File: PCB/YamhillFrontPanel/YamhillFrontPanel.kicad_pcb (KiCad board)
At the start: 2 copper layers, 110 x 50 mm, 6 parts

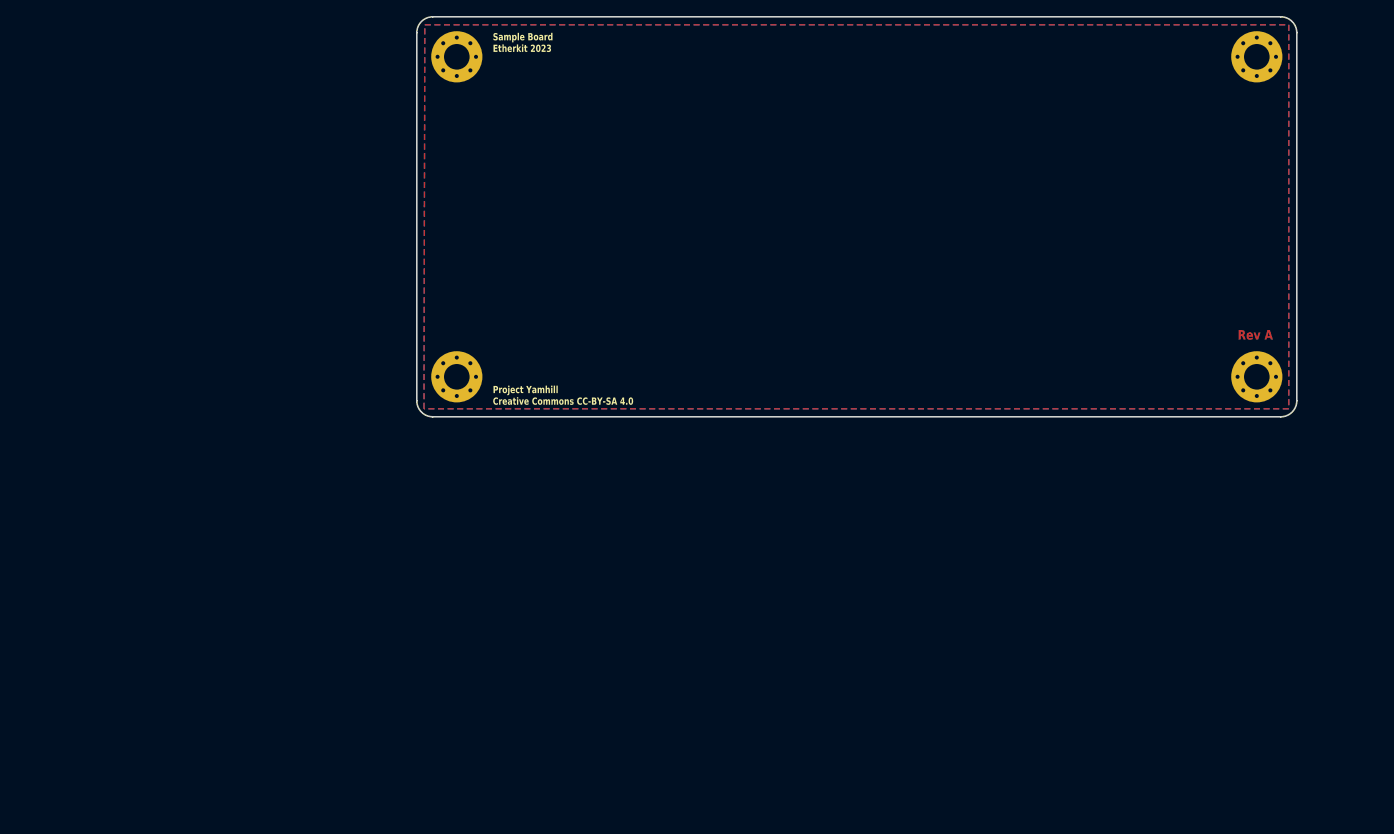
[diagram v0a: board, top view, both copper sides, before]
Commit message: Rev A Front Panel
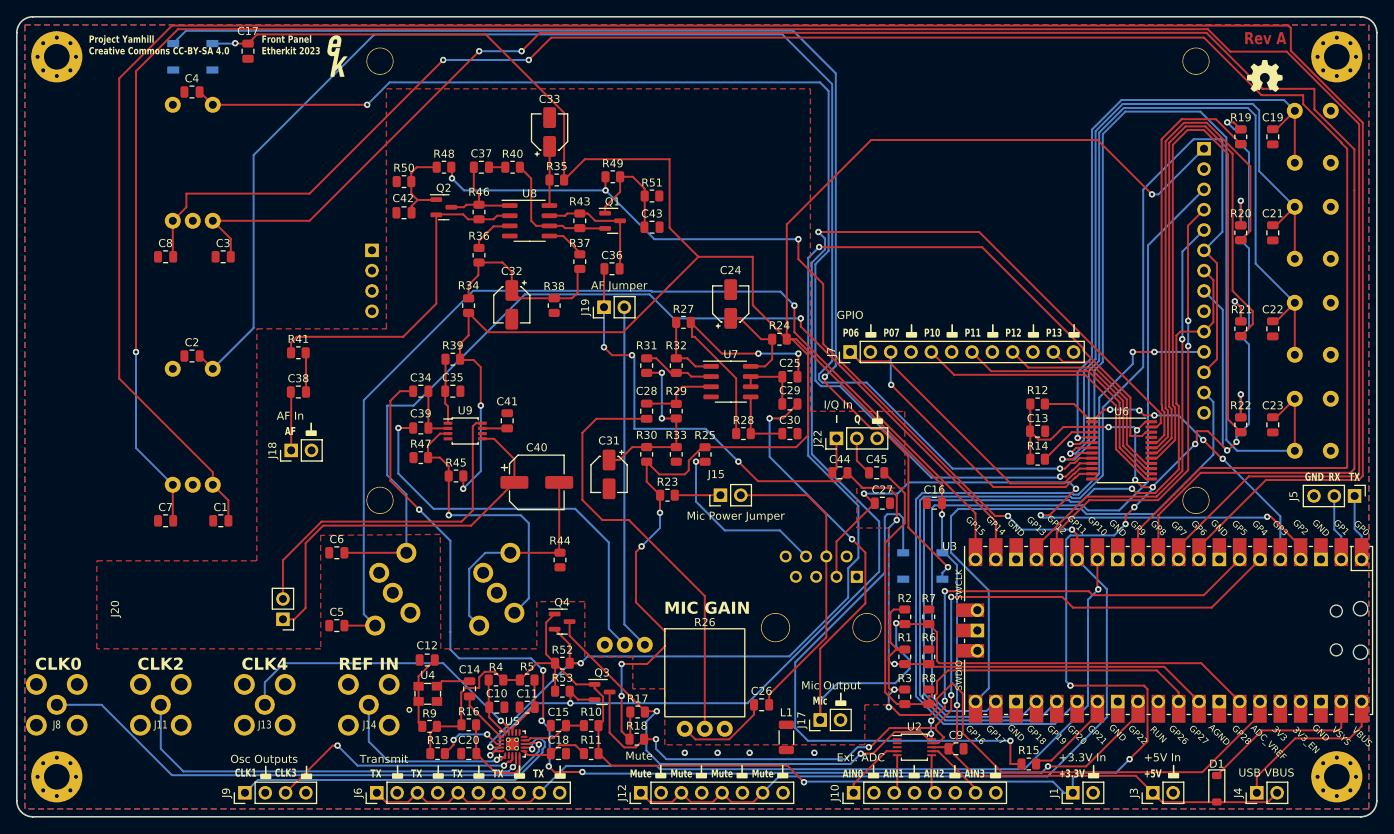
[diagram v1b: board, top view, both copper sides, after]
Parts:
- added C1: 100n, Capacitor_SMD:C_0805_2012Metric, F.Cu at (75.5, 113.0)
- added C10: 100n, Capacitor_SMD:C_0805_2012Metric, F.Cu at (110.0, 136.3)
- added C11: 100n, Capacitor_SMD:C_0805_2012Metric, F.Cu at (113.8, 136.3)
- added C12: 100n, Capacitor_SMD:C_0805_2012Metric, F.Cu at (101.3, 130.4)
- added C13: 100n, Capacitor_SMD:C_0805_2012Metric, F.Cu at (177.6, 101.8)
- added C14: 10n, Capacitor_SMD:C_0805_2012Metric, F.Cu at (106.6, 134.0)
- added C15: 100n, Capacitor_SMD:C_0805_2012Metric, F.Cu at (117.7, 138.6)
- added C16: 100n, Capacitor_SMD:C_0805_2012Metric, F.Cu at (164.7, 110.8)
- added C17: 100n, Capacitor_SMD:C_0805_2012Metric, F.Cu at (78.9, 54.3)
- added C18: 100n, Capacitor_SMD:C_0805_2012Metric, F.Cu at (117.7, 142.1)
- added C19: 100n, Capacitor_SMD:C_0805_2012Metric, F.Cu at (207.0, 65.0)
- added C2: 100n, Capacitor_SMD:C_0805_2012Metric, F.Cu at (71.9, 92.4)
- added C20: 100n, Capacitor_SMD:C_0805_2012Metric, F.Cu at (106.5, 142.1)
- added C21: 100n, Capacitor_SMD:C_0805_2012Metric, F.Cu at (207.0, 77.0)
- added C22: 100n, Capacitor_SMD:C_0805_2012Metric, F.Cu at (207.0, 89.0)
- added C23: 100n, Capacitor_SMD:C_0805_2012Metric, F.Cu at (207.0, 101.0)
- added C24: 10u, Capacitor_SMD:CP_Elec_4x4.5, F.Cu at (139.2, 85.9)
- added C25: 10n, Capacitor_SMD:C_0805_2012Metric, F.Cu at (146.6, 95.0)
- added C26: 1u, Capacitor_SMD:C_0805_2012Metric, F.Cu at (143.1, 136.0)
- added C27: 100n, Capacitor_SMD:C_0805_2012Metric, F.Cu at (158.2, 110.8)
- added C28: 1u, Capacitor_SMD:C_0805_2012Metric, F.Cu at (128.7, 99.3)
- added C29: 1u, Capacitor_SMD:C_0805_2012Metric, F.Cu at (146.6, 98.4)
- added C3: 100n, Capacitor_SMD:C_0805_2012Metric, F.Cu at (75.8, 80.0)
- added C30: 2.7n, Capacitor_SMD:C_0805_2012Metric, F.Cu at (146.6, 102.1)
- added C31: 10u, Capacitor_SMD:CP_Elec_4x4.5, F.Cu at (124.0, 107.2)
- added C32: 10u, Capacitor_SMD:CP_Elec_4x4.5, F.Cu at (111.9, 86.0)
- added C33: 10u, Capacitor_SMD:CP_Elec_4x4.5, F.Cu at (116.6, 64.4)
- added C34: 100n, Capacitor_SMD:C_0805_2012Metric, F.Cu at (100.5, 96.8)
- added C35: 1u, Capacitor_SMD:C_0805_2012Metric, F.Cu at (104.5, 96.8)
- added C36: 1u, Capacitor_SMD:C_0805_2012Metric, F.Cu at (124.4, 81.5)
- added C37: 1u, Capacitor_SMD:C_0805_2012Metric, F.Cu at (108.1, 68.8)
- added C38: 1u, Capacitor_SMD:C_0805_2012Metric, F.Cu at (85.2, 96.9)
- added C39: 100n, Capacitor_SMD:C_0805_2012Metric, F.Cu at (100.5, 101.4)
- added C4: 100n, Capacitor_SMD:C_0805_2012Metric, F.Cu at (71.9, 59.4)
- added C40: 100u, Capacitor_SMD:CP_Elec_6.3x5.9, F.Cu at (115.0, 108.2)
- added C41: 1u, Capacitor_SMD:C_0805_2012Metric, F.Cu at (111.3, 100.5)
- added C42: 1u, Capacitor_SMD:C_0805_2012Metric, F.Cu at (98.4, 74.5)
- added C43: 1u, Capacitor_SMD:C_0805_2012Metric, F.Cu at (129.4, 76.3)
- added C44: 100n, Capacitor_SMD:C_0805_2012Metric, F.Cu at (152.9, 107.0)
- added C45: 100n, Capacitor_SMD:C_0805_2012Metric, F.Cu at (157.5, 107.0)
- added C5: 100n, Capacitor_SMD:C_0805_2012Metric, F.Cu at (90.0, 126.1)
- added C6: 100n, Capacitor_SMD:C_0805_2012Metric, F.Cu at (90.0, 117.0)
- added C7: 100n, Capacitor_SMD:C_0805_2012Metric, F.Cu at (68.6, 113.0)
- added C8: 100n, Capacitor_SMD:C_0805_2012Metric, F.Cu at (68.6, 80.0)
- added C9: 100n, Capacitor_SMD:C_0805_2012Metric, F.Cu at (167.4, 141.5)
- added D1: MBRX120LF-TP, Diode_SMD:D_SOD-123, F.Cu at (200.0, 146.5)
- added D2: WS2812B, LED_SMD:LED_WS2812B_PLCC4_5.0x5.0mm_P3.2mm, B.Cu at (163.2, 118.7)
- added D3: WS2812B, LED_SMD:LED_WS2812B_PLCC4_5.0x5.0mm_P3.2mm, B.Cu at (72.0, 55.0)
- added D4: LED, LED_SMD:LED_0805_2012Metric, B.Cu at (203.0, 65.0)
- added D5: LED, LED_SMD:LED_0805_2012Metric, B.Cu at (203.0, 77.0)
- added D6: LED, LED_SMD:LED_0805_2012Metric, B.Cu at (203.0, 89.0)
- added D7: LED, LED_SMD:LED_0805_2012Metric, B.Cu at (203.0, 101.0)
- added J1: +3.3V In, Connector_PinHeader_2.54mm:PinHeader_1x02_P2.54mm_Vertical, F.Cu at (182.0, 147.0)
- added J10: Ext. ADC, Connector_PinHeader_2.54mm:PinHeader_1x08_P2.54mm_Vertical, F.Cu at (154.6, 147.0)
- added J11: CLK2, EtherkitKicadLibrary:SMA_Jack_Vertical, F.Cu at (68.0, 136.0)
- added J12: Mute, Connector_PinHeader_2.54mm:PinHeader_1x08_P2.54mm_Vertical, F.Cu at (128.0, 147.0)
- added J13: CLK4, EtherkitKicadLibrary:SMA_Jack_Vertical, F.Cu at (81.0, 136.0)
- added J14: REF_IN, EtherkitKicadLibrary:SMA_Jack_Vertical, F.Cu at (94.0, 136.0)
- added J15: Mic Power Jumper, Connector_PinHeader_2.54mm:PinHeader_1x02_P2.54mm_Vertical, F.Cu at (138.0, 109.8)
- added J16: Microphone, Connector_RJ:RJ45_OST_PJ012-8P8CX_Vertical, B.Cu at (155.0, 120.0)
- added J17: Mic Output, Connector_PinHeader_2.54mm:PinHeader_1x02_P2.54mm_Vertical, F.Cu at (150.4, 137.9)
- added J18: AF In, Connector_PinHeader_2.54mm:PinHeader_1x02_P2.54mm_Vertical, F.Cu at (84.3, 104.2)
- added J19: AF Jumper, Connector_PinHeader_2.54mm:PinHeader_1x02_P2.54mm_Vertical, F.Cu at (123.4, 86.3)
- added J2: Paddles, EtherkitKicadLibrary:Kycon_STX-3680-5NB, B.Cu at (97.0, 122.0)
- added J20: Speaker, EtherkitKicadLibrary:Ole_Wolff_OWS-091630W50A-8, F.Cu at (70.0, 124.0)
- added J21: Headphones, EtherkitKicadLibrary:Kycon_STX-3680-5NB, B.Cu at (110.0, 122.0)
- added J22: I/Q In, Connector_PinHeader_2.54mm:PinHeader_1x03_P2.54mm_Vertical, F.Cu at (152.5, 102.7)
- added J3: +5V In, Connector_PinHeader_2.54mm:PinHeader_1x02_P2.54mm_Vertical, F.Cu at (192.0, 147.0)
- added J4: USB VBUS, Connector_PinHeader_2.54mm:PinHeader_1x02_P2.54mm_Vertical, F.Cu at (205.0, 147.0)
- added J5: UART, Connector_PinHeader_2.54mm:PinHeader_1x03_P2.54mm_Vertical, F.Cu at (217.2, 109.9)
- added J6: Transmit, Connector_PinHeader_2.54mm:PinHeader_1x10_P2.54mm_Vertical, F.Cu at (95.0, 147.0)
- added J7: GPIO, Connector_PinHeader_2.54mm:PinHeader_1x12_P2.54mm_Vertical, F.Cu at (154.2, 91.9)
- added J8: CLK0, EtherkitKicadLibrary:SMA_Jack_Vertical, F.Cu at (55.0, 136.0)
- added J9: Osc Outputs, Connector_PinHeader_2.54mm:PinHeader_1x04_P2.54mm_Vertical, F.Cu at (78.5, 147.0)
- added L1: Fair-Rite 2512066017Y1, Inductor_SMD:L_1206_3216Metric, F.Cu at (146.2, 140.1)
- added Q1: 2N7002, Package_TO_SOT_SMD:SOT-23, F.Cu at (124.5, 75.5)
- added Q2: 2N7002, Package_TO_SOT_SMD:SOT-23, F.Cu at (103.4, 73.8)
- added Q3: 2N7002, Package_TO_SOT_SMD:SOT-23, F.Cu at (123.2, 134.4)
- added Q4: 2N7002, Package_TO_SOT_SMD:SOT-23, F.Cu at (118.2, 125.6)
- added R1: 47k, Resistor_SMD:R_0805_2012Metric, F.Cu at (161.0, 130.0)
- added R10: 47, Resistor_SMD:R_0805_2012Metric, F.Cu at (121.8, 138.6)
- added R11: 47, Resistor_SMD:R_0805_2012Metric, F.Cu at (121.8, 142.1)
- added R12: 10k, Resistor_SMD:R_0805_2012Metric, F.Cu at (177.6, 98.4)
- added R13: 10k, Resistor_SMD:R_0805_2012Metric, F.Cu at (102.6, 142.1)
- added R14: 10k, Resistor_SMD:R_0805_2012Metric, F.Cu at (177.6, 105.3)
- added R15: 470, Resistor_SMD:R_0805_2012Metric, F.Cu at (176.5, 143.4)
- added R16: 47, Resistor_SMD:R_0805_2012Metric, F.Cu at (106.5, 138.5)
- added R17: 4.7k, Resistor_SMD:R_0805_2012Metric, F.Cu at (127.6, 136.9)
- added R18: 4.7k, Resistor_SMD:R_0805_2012Metric, F.Cu at (127.5, 140.3)
- added R19: 330, Resistor_SMD:R_0805_2012Metric, F.Cu at (203.0, 65.0)
- added R2: 47k, Resistor_SMD:R_0805_2012Metric, F.Cu at (161.0, 125.0)
- added R20: 330, Resistor_SMD:R_0805_2012Metric, F.Cu at (203.0, 77.0)
- added R21: 330, Resistor_SMD:R_0805_2012Metric, F.Cu at (203.0, 89.0)
- added R22: 330, Resistor_SMD:R_0805_2012Metric, F.Cu at (203.0, 101.0)
- added R23: 7.5k, Resistor_SMD:R_0805_2012Metric, F.Cu at (131.3, 109.8)
- added R24: 47, Resistor_SMD:R_0805_2012Metric, F.Cu at (145.3, 90.3)
- added R25: 470, Resistor_SMD:R_0805_2012Metric, F.Cu at (136.0, 104.7)
- added R26: 5k trim, EtherkitKicadLibrary:Bournes_PTV09A, F.Cu at (136.0, 132.0)
- added R27: 10k, Resistor_SMD:R_0805_2012Metric, F.Cu at (133.3, 88.2)
- added R28: 10k, Resistor_SMD:R_0805_2012Metric, F.Cu at (140.8, 102.1)
- added R29: 100k, Resistor_SMD:R_0805_2012Metric, F.Cu at (132.4, 99.3)
- added R3: 47k, Resistor_SMD:R_0805_2012Metric, F.Cu at (161.0, 135.0)
- added R30: 10k, Resistor_SMD:R_0805_2012Metric, F.Cu at (128.7, 104.7)
- added R31: 470, Resistor_SMD:R_0805_2012Metric, F.Cu at (128.7, 93.6)
- added R32: 270k, Resistor_SMD:R_0805_2012Metric, F.Cu at (132.4, 93.6)
- added R33: 10k, Resistor_SMD:R_0805_2012Metric, F.Cu at (132.4, 104.7)
- added R34: 10k, Resistor_SMD:R_0805_2012Metric, F.Cu at (106.5, 86.1)
- added R35: 47, Resistor_SMD:R_0805_2012Metric, F.Cu at (117.5, 70.4)
- added R36: 100k, Resistor_SMD:R_0805_2012Metric, F.Cu at (107.8, 79.8)
- added R37: 100k, Resistor_SMD:R_0805_2012Metric, F.Cu at (120.4, 80.6)
- added R38: 10k, Resistor_SMD:R_0805_2012Metric, F.Cu at (117.2, 86.1)
- added R39: 47, Resistor_SMD:R_0805_2012Metric, F.Cu at (104.5, 92.8)
- added R4: 47, Resistor_SMD:R_0805_2012Metric, F.Cu at (109.9, 132.9)
- added R40: 1k, Resistor_SMD:R_0805_2012Metric, F.Cu at (112.0, 68.8)
- added R41: 100, Resistor_SMD:R_0805_2012Metric, F.Cu at (85.2, 92.0)
- added R42: 10k, EtherkitKicadLibrary:Alps_RK09L1140, B.Cu at (126.0, 122.0)
- added R43: 10k, Resistor_SMD:R_0805_2012Metric, F.Cu at (120.4, 75.5)
- added R44: 150, Resistor_SMD:R_0805_2012Metric, F.Cu at (117.9, 117.9)
- added R45: 100k, Resistor_SMD:R_0805_2012Metric, F.Cu at (104.9, 107.4)
- added R46: 1k, Resistor_SMD:R_0805_2012Metric, F.Cu at (107.8, 74.4)
- added R47: 100k, Resistor_SMD:R_0805_2012Metric, F.Cu at (100.5, 105.1)
- added R48: 470, Resistor_SMD:R_0805_2012Metric, F.Cu at (103.4, 68.8)
- added R49: 1k, Resistor_SMD:R_0805_2012Metric, F.Cu at (124.5, 70.0)
- added R5: 47, Resistor_SMD:R_0805_2012Metric, F.Cu at (113.8, 132.9)
- added R50: 100k, Resistor_SMD:R_0805_2012Metric, F.Cu at (98.4, 70.6)
- added R51: 100k, Resistor_SMD:R_0805_2012Metric, F.Cu at (129.4, 72.4)
- added R52: 4.7k, Resistor_SMD:R_0805_2012Metric, F.Cu at (118.2, 130.8)
- added R53: 4.7k, Resistor_SMD:R_0805_2012Metric, F.Cu at (118.2, 134.3)
- added R6: 47k, Resistor_SMD:R_0805_2012Metric, F.Cu at (164.0, 130.0)
- added R7: 47k, Resistor_SMD:R_0805_2012Metric, F.Cu at (164.0, 125.0)
- added R8: 47k, Resistor_SMD:R_0805_2012Metric, F.Cu at (164.0, 135.0)
- added R9: 47, Resistor_SMD:R_0805_2012Metric, F.Cu at (101.6, 138.7)
- added S1: PUSHBUTTON_TACTILE, EtherkitKicadLibrary:E-Switch_TL1105, B.Cu at (212.0, 65.0)
- added S2: PUSHBUTTON_TACTILE, EtherkitKicadLibrary:E-Switch_TL1105, B.Cu at (212.0, 77.0)
- added S3: PUSHBUTTON_TACTILE, EtherkitKicadLibrary:E-Switch_TL1105, B.Cu at (212.0, 89.0)
- added S4: PUSHBUTTON_TACTILE, EtherkitKicadLibrary:E-Switch_TL1105, B.Cu at (212.0, 101.0)
- added SW1: Tune, EtherkitKicadLibrary:Bournes_PEC11R-4xxxF-Sxxxx, B.Cu at (72.0, 101.0)
- added SW2: Multifunction, EtherkitKicadLibrary:Bournes_PEC11R-4xxxF-Sxxxx, B.Cu at (72.0, 68.0)
- added U1: 4" TFT LCD ST7796S, EtherkitKicadLibrary:ST7796_4.0in, B.Cu at (146.4, 83.0)
- added U2: ADS1115IDGS, Package_SO:TSSOP-10_3x3mm_P0.5mm, F.Cu at (162.2, 141.3)
- added U3: Pico, MCU_RaspberryPi_and_Boards:RPi_Pico_SMD_TH, F.Cu at (194.0, 126.7)
- added U4: ATX-H11-F-25.000MHZ-F25-T, EtherkitKicadLibrary:ASTX-H11-25.000MHZ-T, F.Cu at (101.4, 134.6)
- added U5: Si5351C, Package_DFN_QFN:VQFN-20-1EP_3x3mm_P0.45mm_EP1.55x1.55mm_ThermalVias, F.Cu at (112.0, 140.9)
- added U6: TCAL6416, Package_SO:TSSOP-24_6.1x7.8mm_P0.65mm, F.Cu at (188.1, 104.2)
- added U7: TLV9362, Package_SO:SOIC-8_3.9x4.9mm_P1.27mm, F.Cu at (139.3, 95.6)
- added U8: TLV9362, Package_SO:SOIC-8_3.9x4.9mm_P1.27mm, F.Cu at (114.1, 75.5)
- added U9: LM4875, Package_SO:TSSOP-8_3x3mm_P0.65mm, F.Cu at (106.0, 101.8)
- G***, Ref**: moved to F.Cu
- moved Ref** 119.5 mm to (90.1, 54.9), turned to 0 degrees
- moved G*** 105.7 mm to (206.0, 57.4), turned to 0 degrees
- moved H3 70.7 mm to (55.0, 145.0)
- moved H4 51.0 mm to (215.0, 145.0)
- moved H1 50.0 mm to (55.0, 55.0)
- moved H2 10.0 mm to (215.0, 55.0)
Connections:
- H1 pad 1: unconnected-(H1-Pad1) -> GNDD
- H2 pad 1: unconnected-(H2-Pad1) -> GNDD
- H3 pad 1: unconnected-(H3-Pad1) -> GNDD
- H4 pad 1: unconnected-(H4-Pad1) -> GNDD
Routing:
- net +5V: track 0.00 -> 431.4 mm, vias 0 -> 10
- net ENC1_A: track 0.00 -> 295.7 mm
- net ENC1_B: track 0.00 -> 289.8 mm, vias 0 -> 1
- net +3.3V: track 0.00 -> 284.7 mm, vias 0 -> 12
- net ENC2_B: track 0.00 -> 241.1 mm, vias 0 -> 2
- net ENC2_A: track 0.00 -> 237.8 mm, vias 0 -> 2
- net MUTE: track 0.00 -> 195.0 mm, vias 0 -> 5
- net ENC1_SW: track 0.00 -> 189.1 mm, vias 0 -> 1
- net SDA_3V3: track 0.00 -> 167.0 mm, vias 0 -> 3
- net SCL_3V3: track 0.00 -> 162.5 mm, vias 0 -> 3
- net ENC2_SW: track 0.00 -> 158.1 mm, vias 0 -> 2
- net Net-(D2-DOUT): track 0.00 -> 156.8 mm, vias 0 -> 2
- net SPI_TX: track 0.00 -> 149.7 mm
- net MCU_DAC: track 0.00 -> 141.5 mm, vias 0 -> 6
- net PDL_B: track 0.00 -> 134.0 mm, vias 0 -> 1
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- added copper zone on F.Cu, net GND
- added copper zone on B.Cu, net GNDD
- added copper zone on F.Cu, net GNDD
- removed copper zone on B.Cu, net (none)
- removed copper zone on F.Cu, net (none)
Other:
- board size 110 x 50 mm -> 170 x 100 mm
- board text added: "+3.3V"
- board text added: "+5V"
- board text added: "AF"
- board text added: "AIN0"
- board text added: "AIN1"
- board text added: "AIN2"
- board text added: "AIN3"
- board text added: "CLK0"
- board text added: "CLK1"
- board text added: "CLK2"
- board text added: "CLK3"
- board text added: "CLK4"
- board text added: "Front Panel Etherkit 2023"
- board text added: "GND"
- board text added: "I"
- board text added: "MIC GAIN"
- board text added: "Mic"
- board text added: "Mute"
- board text added: "P06"
- board text added: "P07"
- board text added: "P10"
- board text added: "P11"
- board text added: "P12"
- board text added: "P13"
- board text added: "Q"
- board text added: "REF IN"
- board text added: "RX"
- board text added: "TX"
- board text removed: "Sample Board Etherkit 2023"
